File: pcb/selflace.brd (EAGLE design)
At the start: 25.4 x 47 mm, 45 parts, among them IC1 78L05Z, J3 AVR_SPI_PROG_3X2NS, U1 ATMEGA328P_TQFP, Y1 16MHz

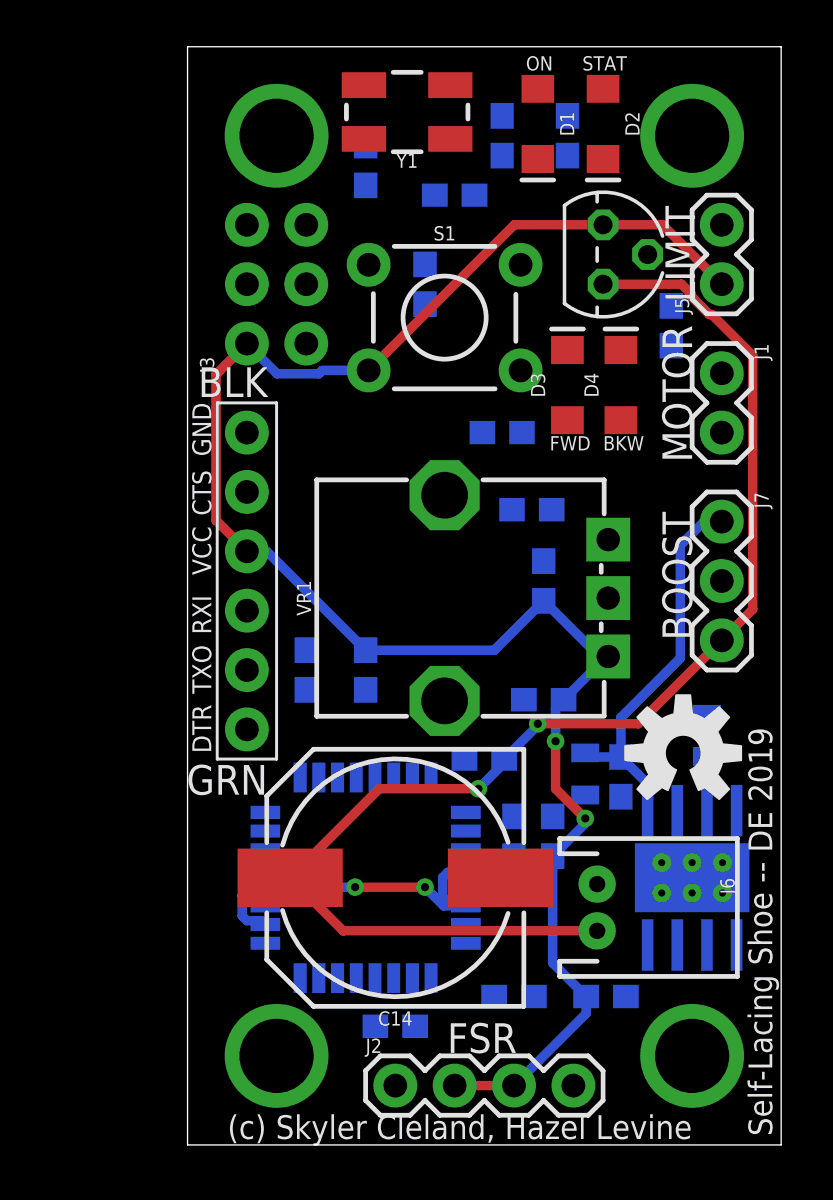
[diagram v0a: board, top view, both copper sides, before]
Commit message: yay, it's a thing that does a thing that's made to do a thing
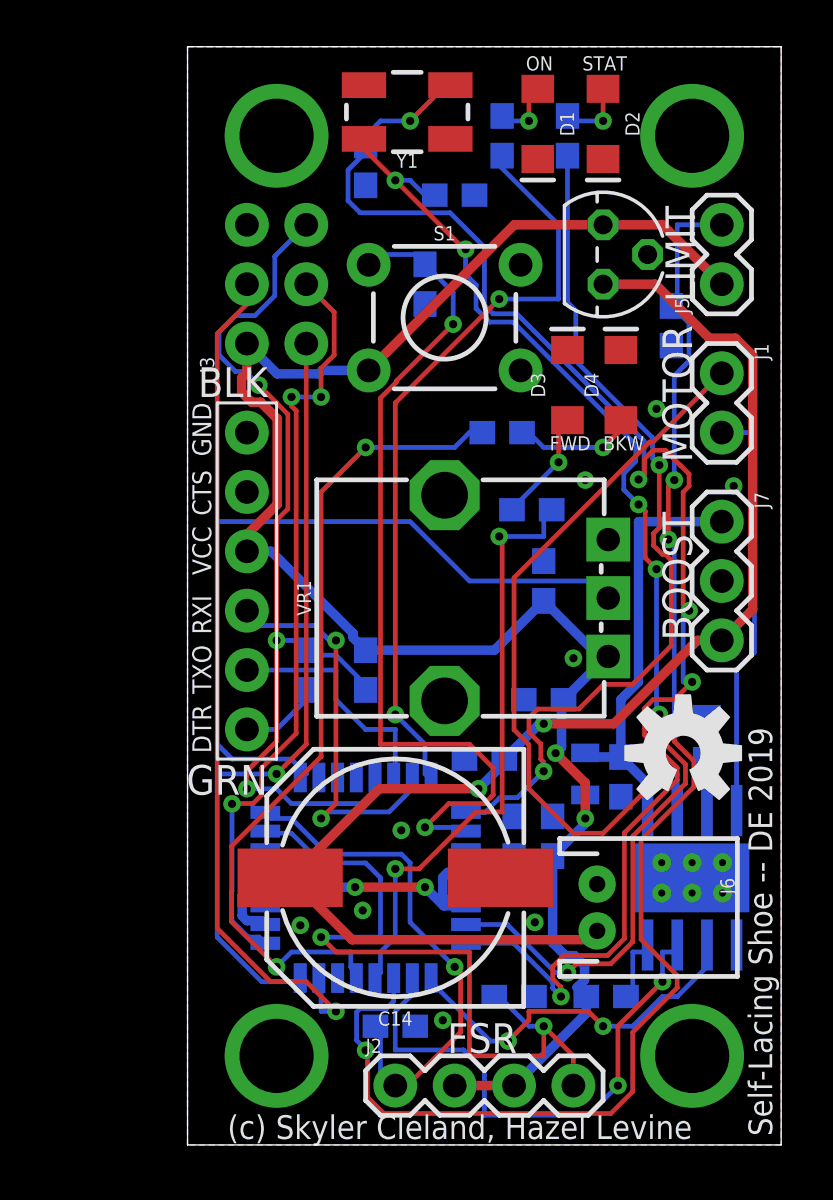
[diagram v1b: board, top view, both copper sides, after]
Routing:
- net N$11: track 0.00 -> 64.9 mm, vias 0 -> 5
- net N$2: track 0.00 -> 61.2 mm, vias 0 -> 4
- net N$7: track 0.00 -> 52.5 mm, vias 0 -> 6
- net RESET: track 0.00 -> 40.2 mm, vias 0 -> 3
- net DIG3: track 0.00 -> 37.1 mm, vias 0 -> 2
- net N$1: track 0.00 -> 37.0 mm, vias 0 -> 2
- net MOSI: track 0.00 -> 36.7 mm, vias 0 -> 1
- net DIG9: track 0.00 -> 35.3 mm, vias 0 -> 2
- net MISO: track 0.00 -> 33.4 mm, vias 0 -> 1
- net SCK: track 0.00 -> 32.8 mm, vias 0 -> 3
- net DIG2: track 0.00 -> 32.7 mm, vias 0 -> 2
- net N$6: track 0.00 -> 32.2 mm
- net N$9: track 0.00 -> 32.0 mm, vias 0 -> 2
- net N$4: track 0.00 -> 31.6 mm, vias 0 -> 1
- net DIG8: track 0.00 -> 26.0 mm, vias 0 -> 2
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- added copper zone on layer 1, net GND
- added copper zone on layer 16, net GND
